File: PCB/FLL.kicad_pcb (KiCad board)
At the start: 2 copper layers, 31.5 x 23.5 mm, 16 parts, among them U2 MCP73831-2-OT, U3 LM317L_SOT-89

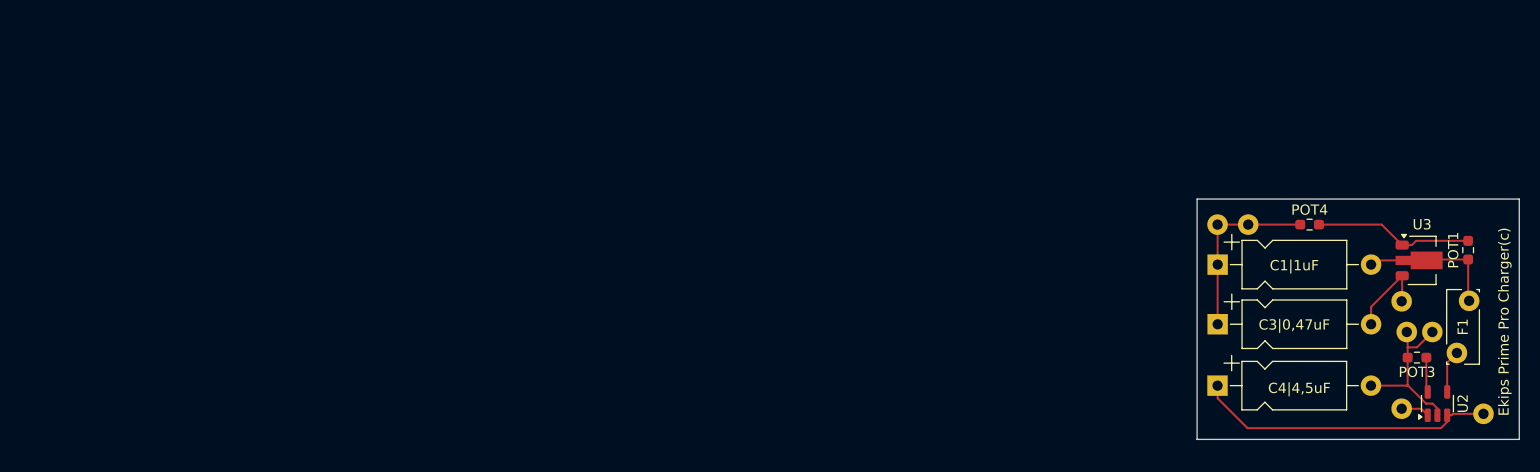
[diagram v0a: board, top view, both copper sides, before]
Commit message: Added Mouser Electronics Parts
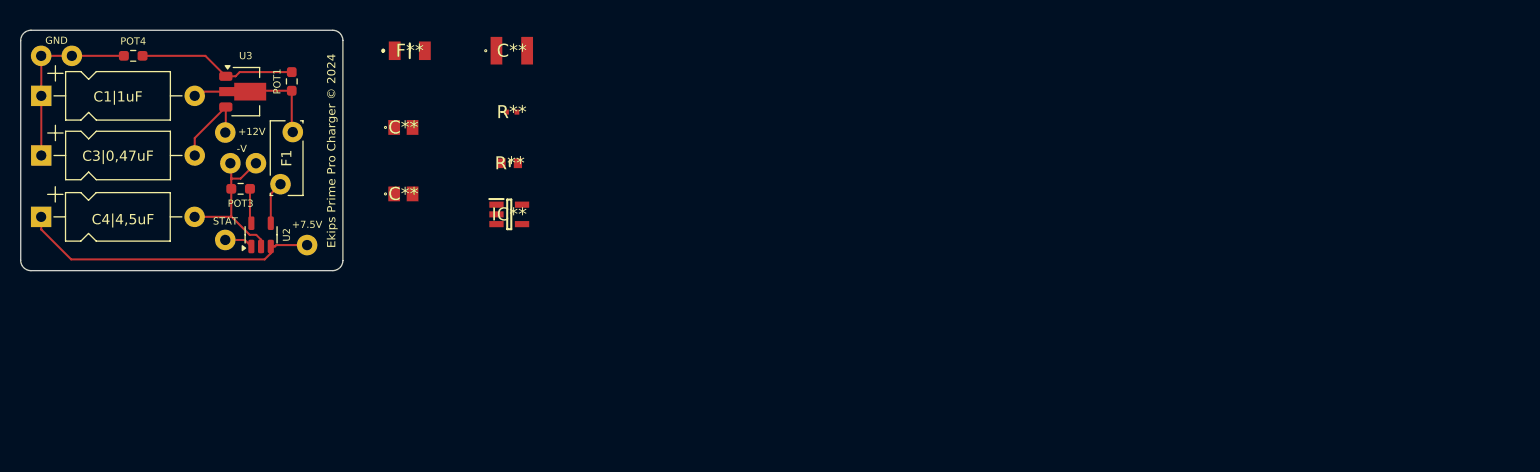
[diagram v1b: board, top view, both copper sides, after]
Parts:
- added C**: C1210, C1210C475K4PACTU_(4.7 uF):C1210, F.Cu at (63.0, 17.0)
- added C**: C0805, C0805C474K5RACTU_(0.47 uF):C0805, F.Cu at (52.4, 31.0)
- added C**: C0805, C0805C105K4RACTU_(1 uF):C0805, F.Cu at (52.4, 24.5)
- added F**: 1206L05015YR, 1206L075THYR_(290 mOhms):1206L05015YR, F.Cu at (53.0, 17.0)
- added IC**: SOT95P270X145-5N, MCP73831T-2ACI/OT:SOT95P270X145-5N, F.Cu at (62.8, 33.0)
- added R**: RESC1608X55N, RC0603FR-071KL_(1 kOhms):RESC1608X55N, F.Cu at (62.8, 28.0)
- added R**: ERJ2RKD1004X, ERJ-2RHD1401X_(1.4 kOhms):ERJ2RKD1004X, F.Cu at (63.0, 23.0)
- moved ? 116.2 mm to (20.0, 17.5)
- moved ? 116.2 mm to (38.0, 28.0)
- moved ? 116.2 mm to (35.5, 28.0)
- moved ? 116.2 mm to (35.0, 25.0)
- moved ? 116.2 mm to (17.0, 17.5)
- moved ? 116.2 mm to (35.0, 35.5)
- moved ? 116.2 mm to (43.0, 36.0)
- moved C4|4,5uF 116.2 mm to (17.0, 33.2)
- moved POT1 116.2 mm to (41.5, 20.0)
- moved POT3 116.2 mm to (36.5, 30.5)
- moved POT4 116.2 mm to (26.0, 17.5)
- moved U2 116.2 mm to (38.5, 35.0)
- moved U3 116.2 mm to (37.0, 21.0)
- moved C1|1uF 116.2 mm to (17.0, 21.4)
- moved C3|0,47uF 116.2 mm to (17.0, 27.2)
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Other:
- outline, holes or cut-outs redrawn
- board text added: "+12V"
- board text added: "+7.5V"
- board text added: "-V"
- board text added: "0.47uF"
- board text added: "1.4kOhms"
- board text added: "1kOhms"
- board text added: "1uF"
- board text added: "290mOhms"
- board text added: "4.7uF"
- board text added: "Ekips Prime Pro Charger © 2024"
- board text added: "GND"
- board text added: "MCP73831T-2ACI/OT"
- board text added: "STAT"
- board text removed: "Ekips Prime Pro Charger(c)"

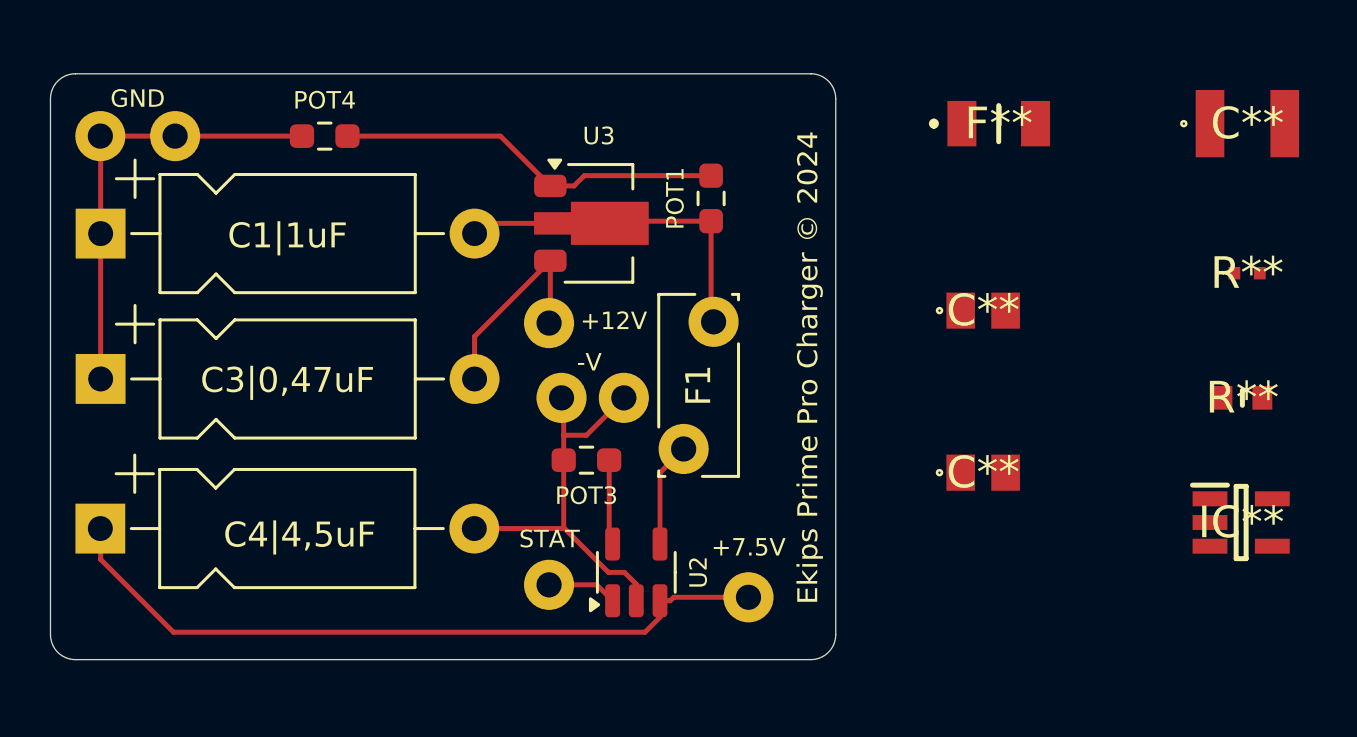
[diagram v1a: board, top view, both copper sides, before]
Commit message: chore: Remove unused KiCad symbol files
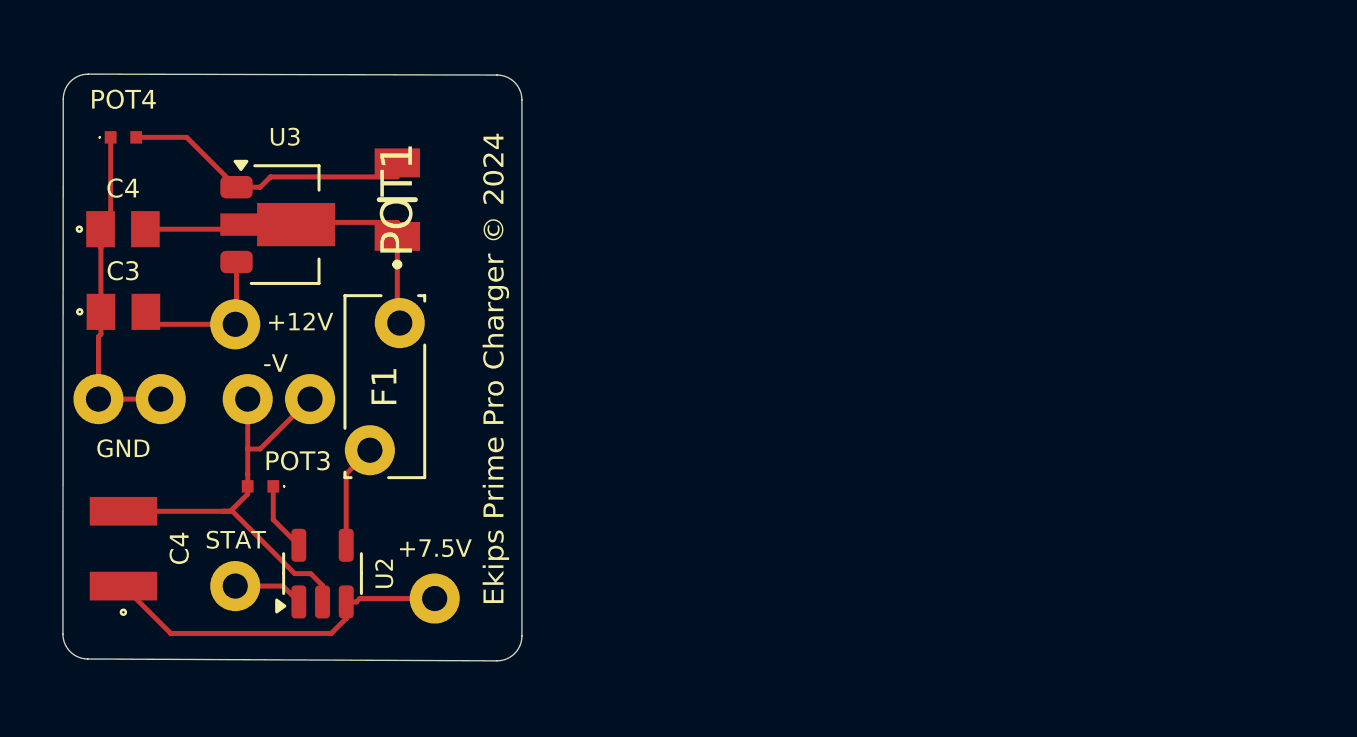
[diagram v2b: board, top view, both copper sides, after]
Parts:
- removed C**: C1210, C1210C475K4PACTU_(4.7 uF):C1210
- removed C**: C0805, C0805C474K5RACTU_(0.47 uF):C0805
- removed C**: C0805, C0805C105K4RACTU_(1 uF):C0805
- removed F**: 1206L05015YR, 1206L075THYR_(290 mOhms):1206L05015YR
- removed IC**: SOT95P270X145-5N, MCP73831T-2ACI/OT:SOT95P270X145-5N
- removed R**: RESC1608X55N, RC0603FR-071KL_(1 kOhms):RESC1608X55N
- removed R**: ERJ2RKD1004X, ERJ-2RHD1401X_(1.4 kOhms):ERJ2RKD1004X
- C3: renamed from C3|0,47uF; footprint Capacitor_THT:CP_Axial_L10.0mm_D4.5mm_P15.00mm_Horizontal -> C0805C474K5RACTU:C0805
- C4: renamed from C4|4,5uF; value 4,5uF -> 4,7uF; footprint Capacitor_THT:CP_Axial_L10.0mm_D4.5mm_P15.00mm_Horizontal -> C1210C475K4PACTU:C1210
- C4: renamed from C1|1uF; footprint Capacitor_THT:CP_Axial_L10.0mm_D4.5mm_P15.00mm_Horizontal -> C0805C105K4RACTU:C0805
- POT1: value 240Ω -> 1206L05015YR; footprint Resistor_SMD:R_0603_1608Metric_Pad0.98x0.95mm_HandSolder -> 1206L075THYR:1206L05015YR
- POT3, POT4: footprint Resistor_SMD:R_0603_1608Metric_Pad0.98x0.95mm_HandSolder -> ERJ-2RHD1401X:ERJ2RKD1004X
- moved POT3 13.1 mm to (23.4, 31.6)
- moved ? 12.6 mm to (25.4, 28.1)
- moved ? 12.6 mm to (22.9, 28.1)
- moved ? 12.6 mm to (22.4, 25.1)
- moved ? 12.6 mm to (22.4, 35.5)
- moved ? 12.6 mm to (30.4, 36.0)
- moved F1 12.6 mm to (29.0, 25.0)
- moved POT1 12.6 mm to (28.9, 20.1)
- moved U2 12.6 mm to (25.9, 35.0)
- moved U3 12.6 mm to (24.4, 21.1)
- moved ? 10.6 mm to (19.4, 28.1)
- moved ? 10.6 mm to (16.9, 28.1)
- moved POT4 8.08 mm to (17.9, 17.6)
- moved C3 2.84 mm to (17.9, 24.6)
- moved C4 1.23 mm to (17.9, 34.0), turned to 90 degrees
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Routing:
- net +7.5V: track 29.8 -> 14.6 mm
- net GND: track 17.9 -> 13.8 mm
- net Net-(U3-ADJ): track 15.6 -> 11.5 mm
- net -7.5V: track 16.4 -> 18.9 mm
- net Net-(U3-VI): track 8.52 -> 7.02 mm
- net Net-(U2-PROG): track 3.42 -> 2.79 mm
- net Net-(U3-VO): track 13.8 -> 14.3 mm
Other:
- board size 31.5 x 23.5 mm -> 18.4 x 23.5 mm
- board text removed: "0.47uF"
- board text removed: "1.4kOhms"
- board text removed: "1kOhms"
- board text removed: "1uF"
- board text removed: "290mOhms"
- board text removed: "4.7uF"
- board text removed: "MCP73831T-2ACI/OT"
